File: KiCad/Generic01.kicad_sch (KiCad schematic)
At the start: 3 parts, among them J1 Header, U1 ESP32-PICO-MINI-02

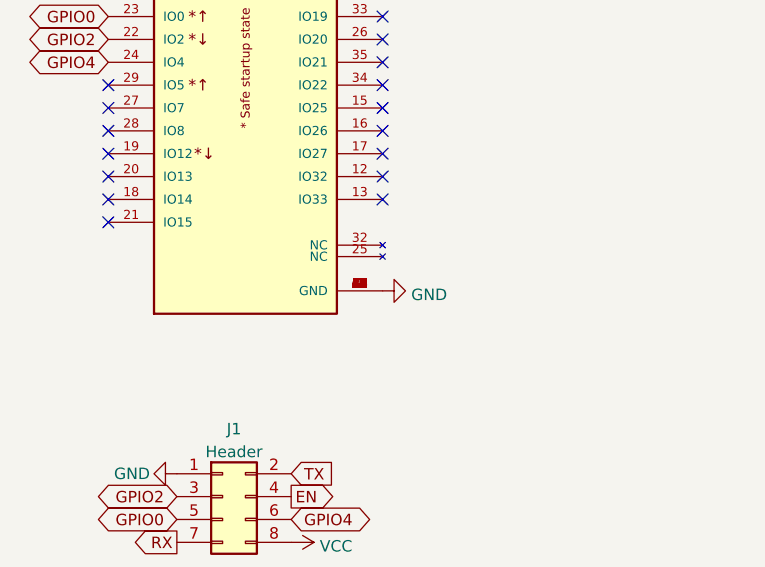
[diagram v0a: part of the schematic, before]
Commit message: Footprint update
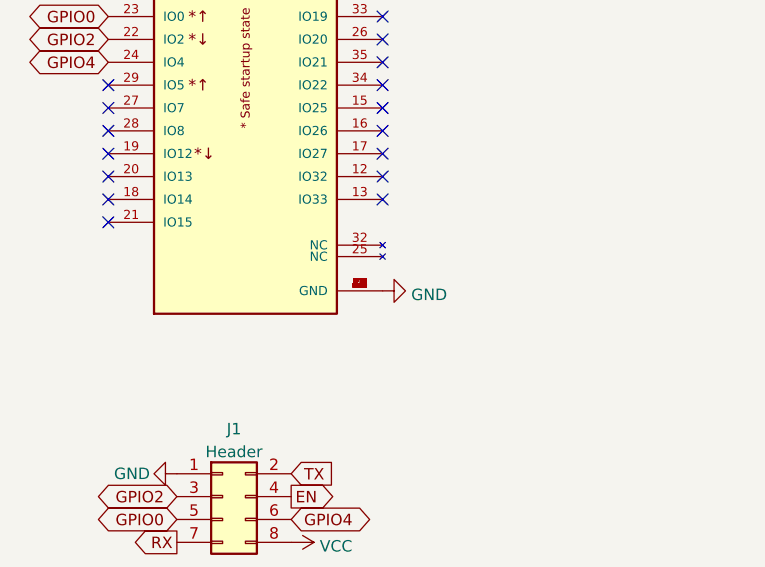
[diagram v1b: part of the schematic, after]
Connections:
- net GND: no longer U1.54 (GND), U1.55 (GND), U1.56 (GND), U1.57 (GND), U1.58 (GND), U1.59 (GND), U1.60 (GND), U1.61 (GND)
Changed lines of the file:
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@@
     (pin "52")
     (pin "53")
-    (pin "54")
-    (pin "55")
-    (pin "56")
-    (pin "57")
-    (pin "58")
-    (pin "59")
     (pin "6")
-    (pin "60")
-    (pin "61")
     (pin "7")
     (pin "8")
